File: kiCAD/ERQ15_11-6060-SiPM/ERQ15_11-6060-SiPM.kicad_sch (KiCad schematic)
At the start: 16 parts, among them J1 Conn, J2 Conn, J3 Conn, J4 Conn, U1 MCP1700x-280xxTT

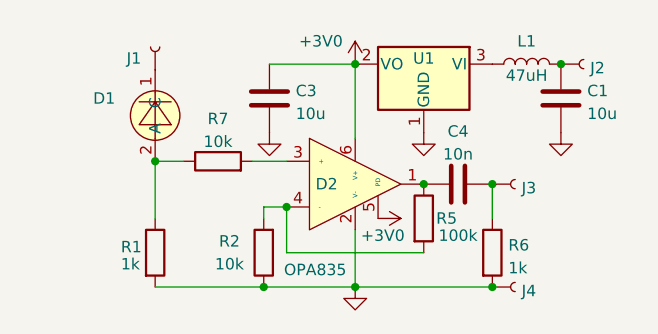
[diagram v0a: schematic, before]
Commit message: изменено:      kiCAD/ERQ15_11-6060-SiPM/ERQ15_11-6060-SiPM.kicad_pcb 	изменено:      kiCAD/ERQ15_11-6060-SiPM/ERQ15_11-6060-SiPM.kicad_prl 	изменено:      kiCAD/ERQ15_11-6060-SiPM/ERQ15_11-6060-SiPM.kicad_pro 	изменено:      kiCAD/ERQ15_11-6060-SiPM/ERQ15_11-6060-SiPM.kicad_sch 	изменено:      kiCAD/ERQ15_11-6060-SiPM/fp-info-cache
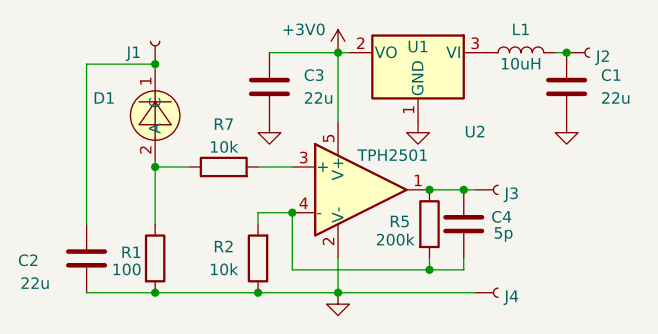
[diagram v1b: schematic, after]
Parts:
- removed D2: OPA835, Package_TO_SOT_SMD:SOT-23-6, symbol My-Library:OPA853
- removed R6: 1k, Resistor_SMD:R_0402_1005Metric, symbol Device:R
- added C2: 22u, Capacitor_SMD:C_1206_3216Metric, symbol Device:C
- added U2: TPH2501, Package_TO_SOT_SMD:SOT-23-5, symbol Amplifier_Operational:OPA356xxDBV
- C1, C3: value 10u -> 22u
- C4: value 10n -> 5p
- L1: value 47uH -> 10uH
- R1: value 1k -> 100
- R5: value 100k -> 200k
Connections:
- net +3V0: now also U2.5 (V+)
- net GND: now also C2.1, U2.2 (V-)
- net at R5.1: now also C4.2, J3.1, U2.1; no longer C4.1
- net at R2.2, R5.2: now also C4.1, U2.4 (-)
- net at D1.1 (C), J1.1: now also C2.2
- net at R7.2: now also U2.3 (+)
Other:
- moved on the sheet: C1, C3, J1, J2, J3, J4, L1, R1, R2, R5, R7, U1
